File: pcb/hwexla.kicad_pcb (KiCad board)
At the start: 4 copper layers, 53.5 x 53 mm, 82 parts, among them J1 DB25_Male, J2 Conn_01x03, J3 AVR-ISP-6, J4 Conn_01x06, J5 Conn_01x04, K1 HFD2/005, Q1 BT148, Q2 2N7002, Q3 2N7002, Q4 2N7002, Q5 2N7002, Q6 2N7002, Q7 BT148, Q8 BT148, SW1 SW_Push, U1 ATmega8A-AU, U2 RR112-1, U3 KA78M05_TO252

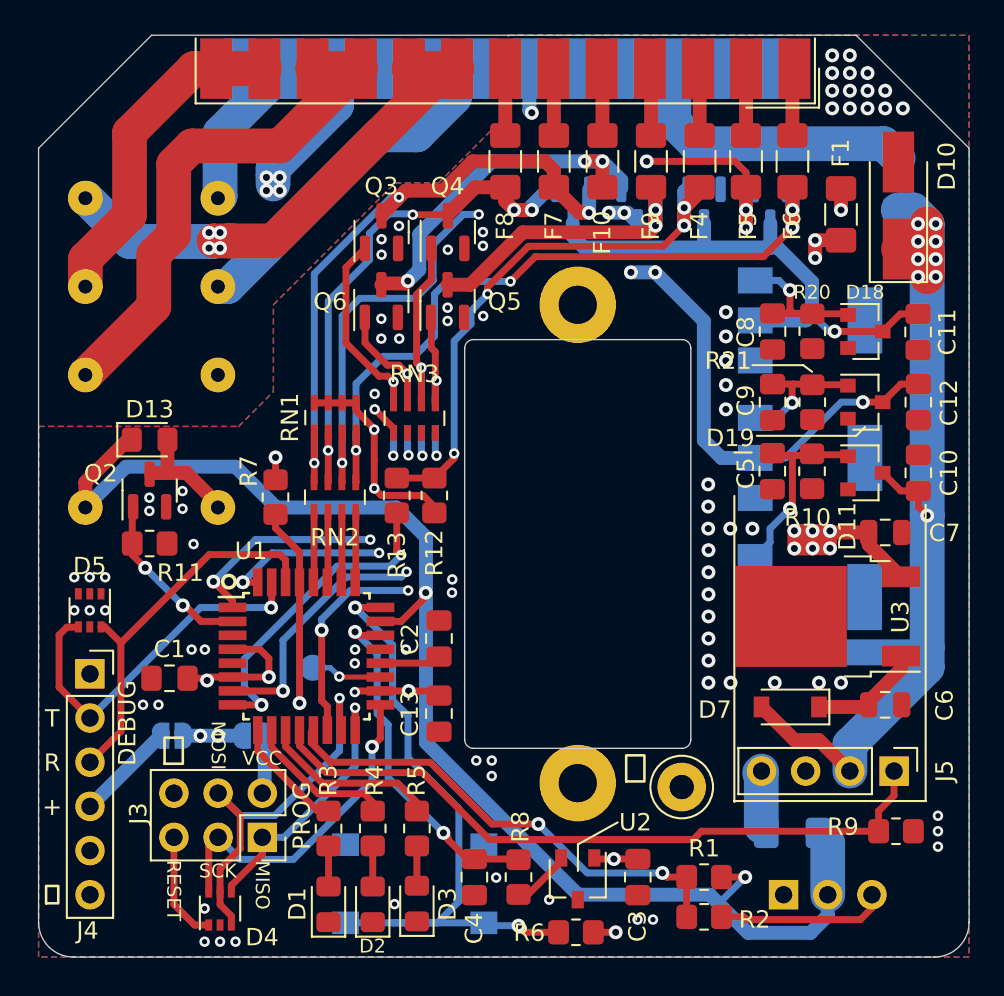
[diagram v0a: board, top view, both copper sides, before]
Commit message: Pcb: power relay from main 5V.
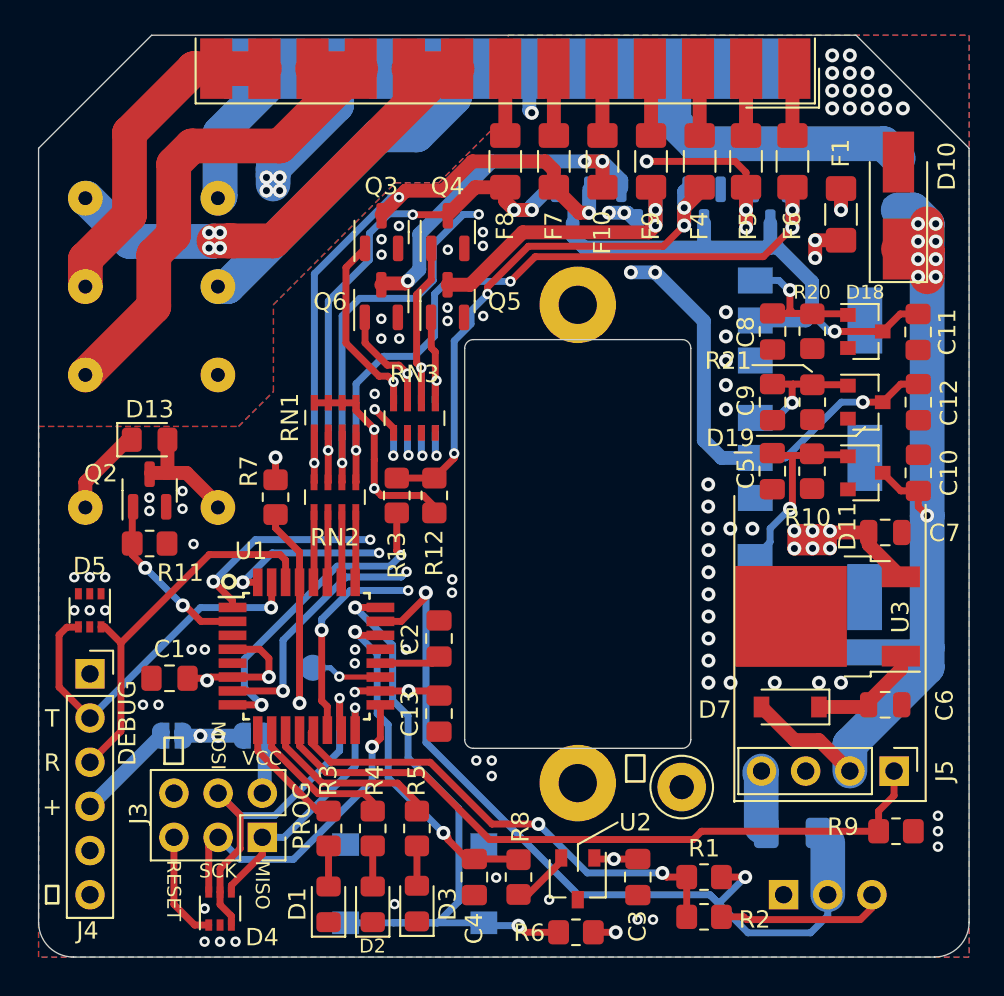
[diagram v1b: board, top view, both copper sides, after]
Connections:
- D13 pad 1: SERVO-VCC -> VCC
- K1 pad 1: SERVO-VCC -> VCC
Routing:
- net SERVO-VCC: track 79.8 -> 49.3 mm
- net VCC: track 51.6 -> 56.7 mm
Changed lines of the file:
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@@
     (fp_line (start -1 0.6) (end 1 0.6) (layer "F.Fab") (width 0.1))
     (pad "1" smd roundrect (at -1.025 0) (size 1.15 1.4) (layers "F.Cu" "F.Paste" "F.Mask") (roundrect_rratio 0.217391)
-      (net 39 "SERVO-VCC") (pinfunction "K") (pintype "passive"))
+      (net 1 "VCC") (pinfunction "K") (pintype "passive"))
     (pad "2" smd roundrect (at 1.025 0) (size 1.15 1.4) (layers "F.Cu" "F.Paste" "F.Mask") (roundrect_rratio 0.217391)
       (net 38 "Net-(D13-Pad2)") (pinfunction "A") (pintype "passive"))
@@
     (fp_line (start 9.398 -5.08) (end -10.922 -5.08) (layer "B.Fab") (width 0.12))
     (pad "1" thru_hole circle (at -9.652 -3.81 90) (size 2 2) (drill 0.8) (layers *.Cu *.Mask)
-      (net 39 "SERVO-VCC") (pintype "passive"))
+      (net 1 "VCC") (pintype "passive"))
     (pad "3" thru_hole circle (at 8.128 -3.81 90) (size 2 2) (drill 0.8) (layers *.Cu *.Mask)
       (net 25 "/RELB-") (pintype "passive"))
@@
   (segment (start 196.088 82.55) (end 196.088 83.566) (width 0.8) (layer "F.Cu") (net 1))
   (segment (start 174.752 80.518) (end 172.339 80.518) (width 0.4) (layer "F.Cu") (net 1))
+  (segment (start 155.324 81.208) (end 155.324 79.753) (width 0.8) (layer "F.Cu") (net 1))
   (segment (start 171.934 76.732) (end 171.934 78.462) (width 0.4) (layer "F.Cu") (net 1))
   (segment (start 197.134 82.556) (end 196.094 82.556) (width 0.8) (layer "F.Cu") (net 1))
@@
   (segment (start 196.088 83.566) (end 197.124 83.566) (width 0.8) (layer "F.Cu") (net 1))
   (segment (start 170.878002 91.758) (end 170.815002 91.821) (width 0.4) (layer "F.Cu") (net 1))
+  (segment (start 157.765 77.312) (end 157.994 77.312) (width 0.8) (layer "F.Cu") (net 1))
   (segment (start 197.134 82.556) (end 197.098 82.556) (width 0.8) (layer "F.Cu") (net 1))
   (segment (start 170.887 75.192) (end 170.887 75.637) (width 0.4) (layer "F.Cu") (net 1))
@@
   (segment (start 175.387 81.153) (end 174.752 80.518) (width 0.4) (layer "F.Cu") (net 1))
   (segment (start 172.339 80.518) (end 171.934 80.113) (width 0.4) (layer "F.Cu") (net 1))
+  (segment (start 155.324 79.753) (end 157.765 77.312) (width 0.8) (layer "F.Cu") (net 1))
   (via (at 173.91 91.758) (size 0.8) (drill 0.4) (layers "F.Cu" "B.Cu") (net 1))
   (via (at 198.134 83.556) (size 0.8) (drill 0.4) (layers "F.Cu" "B.Cu") (net 1))
@@
   (segment (start 191.896 102.458) (end 193.263 102.458) (width 0.4) (layer "F.Cu") (net 39))
   (segment (start 172.286 87.758) (end 173.486 87.758) (width 0.4) (layer "F.Cu") (net 39))
-  (segment (start 155.324 81.208) (end 155.324 79.753) (width 0.8) (layer "F.Cu") (net 39))
   (segment (start 174.894 86.35) (end 174.894 86.105998) (width 0.4) (layer "F.Cu") (net 39))
-  (segment (start 157.765 77.312) (end 157.994 77.312) (width 0.8) (layer "F.Cu") (net 39))
-  (segment (start 155.324 79.753) (end 157.765 77.312) (width 0.8) (layer "F.Cu") (net 39))
   (via (at 193.263 102.458) (size 0.8) (drill 0.4) (layers "F.Cu" "B.Cu") (net 39))
   (via (at 174.894 86.105998) (size 0.8) (drill 0.4) (layers "F.Cu" "B.Cu") (net 39))
-  (segment (start 198.008 104.676081) (end 198.008 103.474) (width 0.8) (layer "B.Cu") (net 39))
-  (segment (start 197.020081 105.664) (end 198.008 104.676081) (width 0.8) (layer "B.Cu") (net 39))
+  (segment (start 198.008 104.676081) (end 198.008 103.474) (width 0.4) (layer "B.Cu") (net 39))
+  (segment (start 191.231 103.474) (end 183.657 103.474) (width 0.4) (layer "B.Cu") (net 39))
+  (segment (start 174.910001 86.121999) (end 174.894 86.105998) (width 0.8) (layer "B.Cu") (net 39))
+  (segment (start 197.020081 105.664) (end 198.008 104.676081) (width 0.4) (layer "B.Cu") (net 39))
   (segment (start 191.643 103.886) (end 191.835 103.886) (width 0.4) (layer "B.Cu") (net 39))
-  (segment (start 183.657 103.474) (end 174.910001 94.727001) (width 0.8) (layer "B.Cu") (net 39))
   (segment (start 191.231 103.474) (end 191.643 103.886) (width 0.4) (layer "B.Cu") (net 39))
   (segment (start 198.008 103.474) (end 198.008 100.4775) (width 2) (layer "B.Cu") (net 39))
-  (segment (start 174.910001 82.916001) (end 173.202 81.208) (width 0.8) (layer "B.Cu") (net 39))
-  (segment (start 173.202 81.208) (end 166.298 81.208) (width 0.8) (layer "B.Cu") (net 39))
-  (segment (start 157.665 78.867) (end 155.324 81.208) (width 0.8) (layer "B.Cu") (net 39))
   (segment (start 198.008 100.4775) (end 197.4485 99.918) (width 1.5) (layer "B.Cu") (net 39))
-  (segment (start 191.231 103.474) (end 183.657 103.474) (width 0.8) (layer "B.Cu") (net 39))
-  (segment (start 163.957 78.867) (end 157.665 78.867) (width 0.8) (layer "B.Cu") (net 39))
-  (segment (start 174.910001 94.727001) (end 174.910001 82.916001) (width 0.8) (layer "B.Cu") (net 39))
   (segment (start 191.835 103.886) (end 193.263 102.458) (width 0.4) (layer "B.Cu") (net 39))
-  (segment (start 193.421 105.664) (end 191.231 103.474) (width 0.8) (layer "B.Cu") (net 39))
-  (segment (start 193.421 105.664) (end 197.020081 105.664) (width 0.8) (layer "B.Cu") (net 39))
-  (segment (start 166.298 81.208) (end 163.957 78.867) (width 0.8) (layer "B.Cu") (net 39))
+  (segment (start 183.657 103.474) (end 174.910001 94.727001) (width 0.4) (layer "B.Cu") (net 39))
+  (segment (start 174.910001 94.727001) (end 174.910001 86.121999) (width 0.4) (layer "B.Cu") (net 39))
+  (segment (start 193.421 105.664) (end 191.231 103.474) (width 0.4) (layer "B.Cu") (net 39))
+  (segment (start 193.421 105.664) (end 197.020081 105.664) (width 0.4) (layer "B.Cu") (net 39))
   (segment (start 195.976 62.7975) (end 195.976 65.12) (width 0.8) (layer "F.Cu") (net 40))
   (segment (start 195.976 64.485) (end 195.976 65.12) (width 0.4) (layer "F.Cu") (net 40))
